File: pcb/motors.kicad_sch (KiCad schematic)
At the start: 4 parts

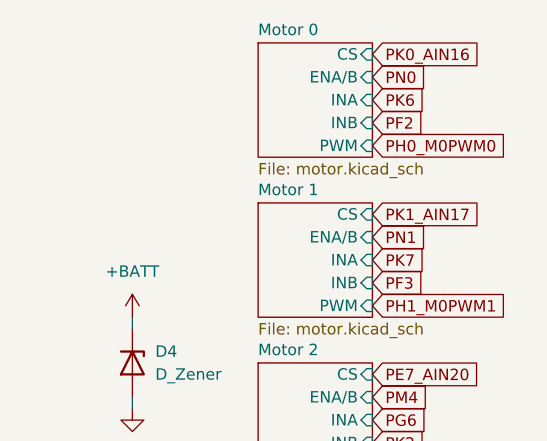
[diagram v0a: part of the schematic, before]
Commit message: Before tear out
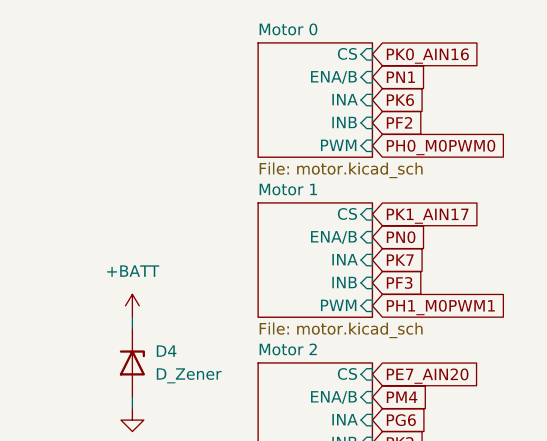
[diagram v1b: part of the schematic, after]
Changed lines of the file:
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@@
 		)
 	)
-	(global_label "PN0"
+	(global_label "PN1"
 		(shape input)
 		(at 179.07 73.66 0)
@@
 		)
 	)
-	(global_label "PN1"
+	(global_label "PN0"
 		(shape input)
 		(at 179.07 91.44 0)
